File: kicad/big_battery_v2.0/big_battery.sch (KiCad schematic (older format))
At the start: 86 parts, among them J1 CN3, J2 CN2, J3 MCU, J4 P1, J5 P0, J6 PRGM, J7 DI, J8 DO, Q1 AO3400, Q2 AO3400, Q3 AO3400, U1 AP1117-ADJ, U2 LMV324, U3 LMV358, U4 EFM8BB10F2G-A-QFN20, U5 PC817, U6 PC817

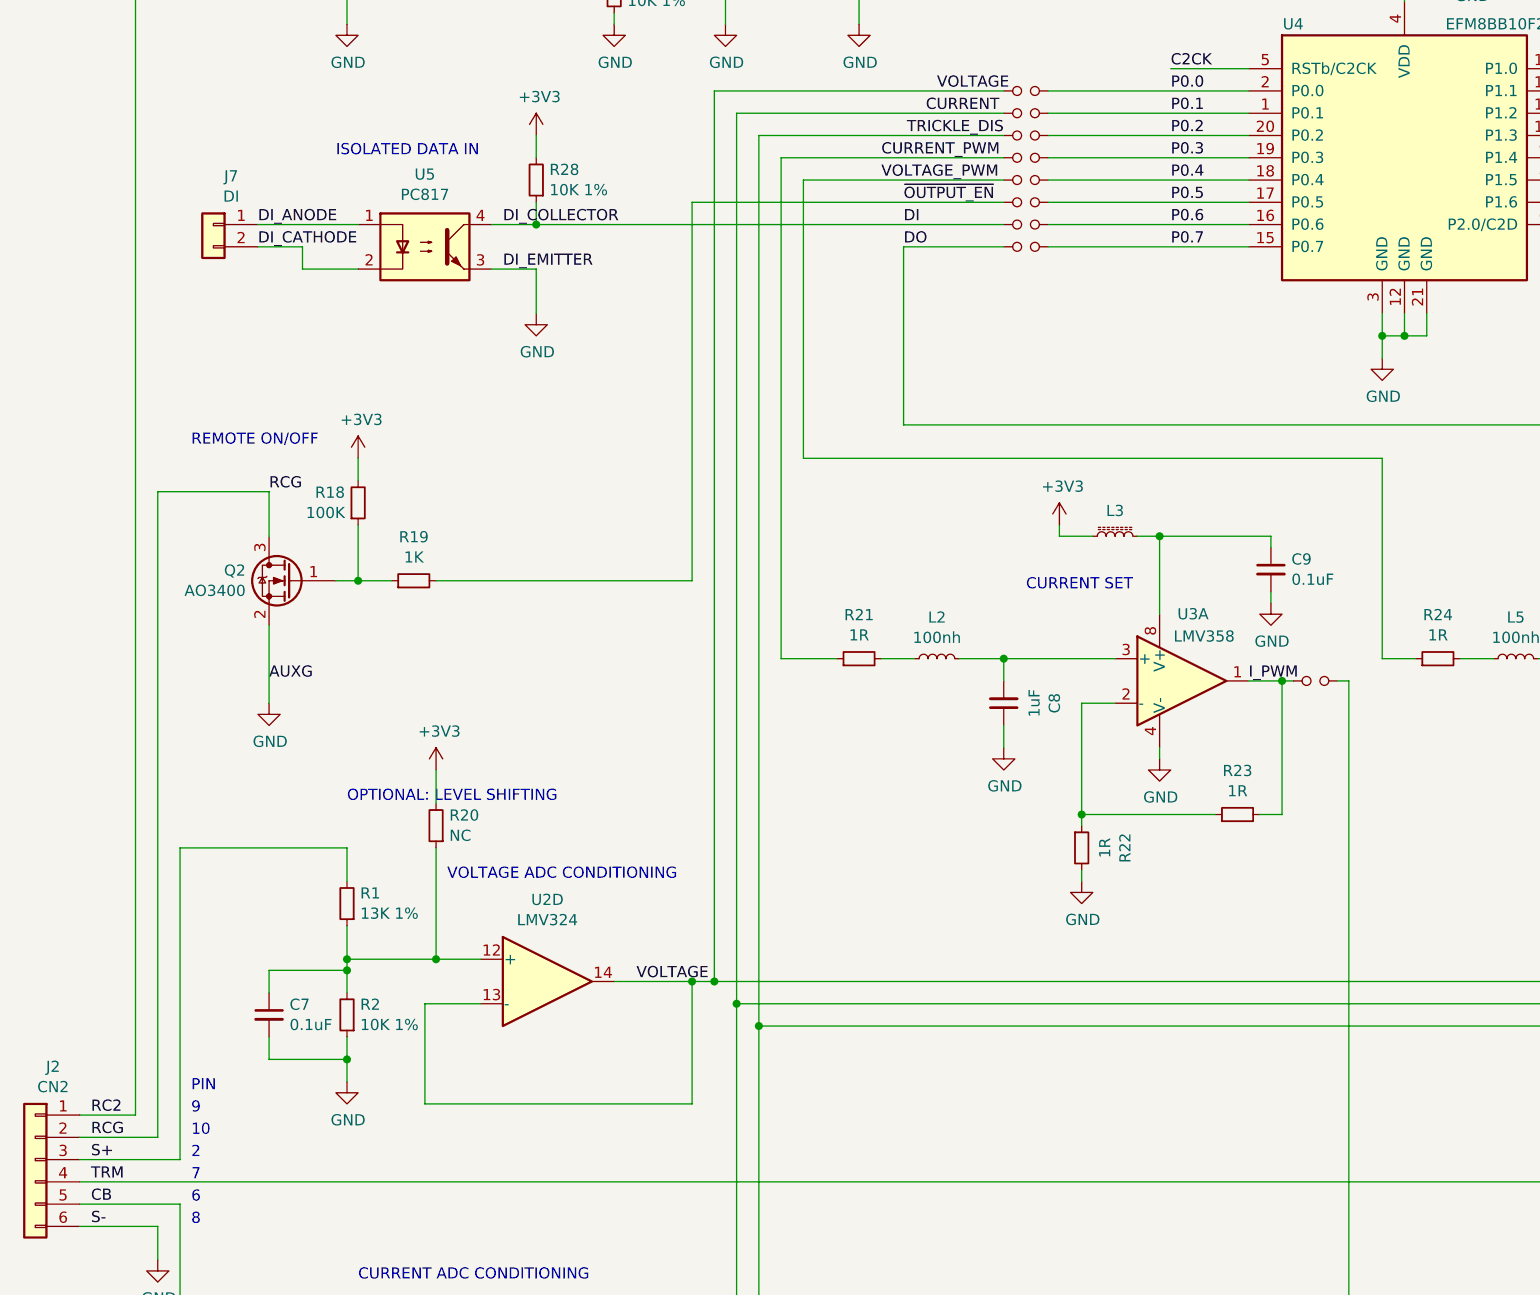
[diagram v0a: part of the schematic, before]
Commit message: final gerbers sent out
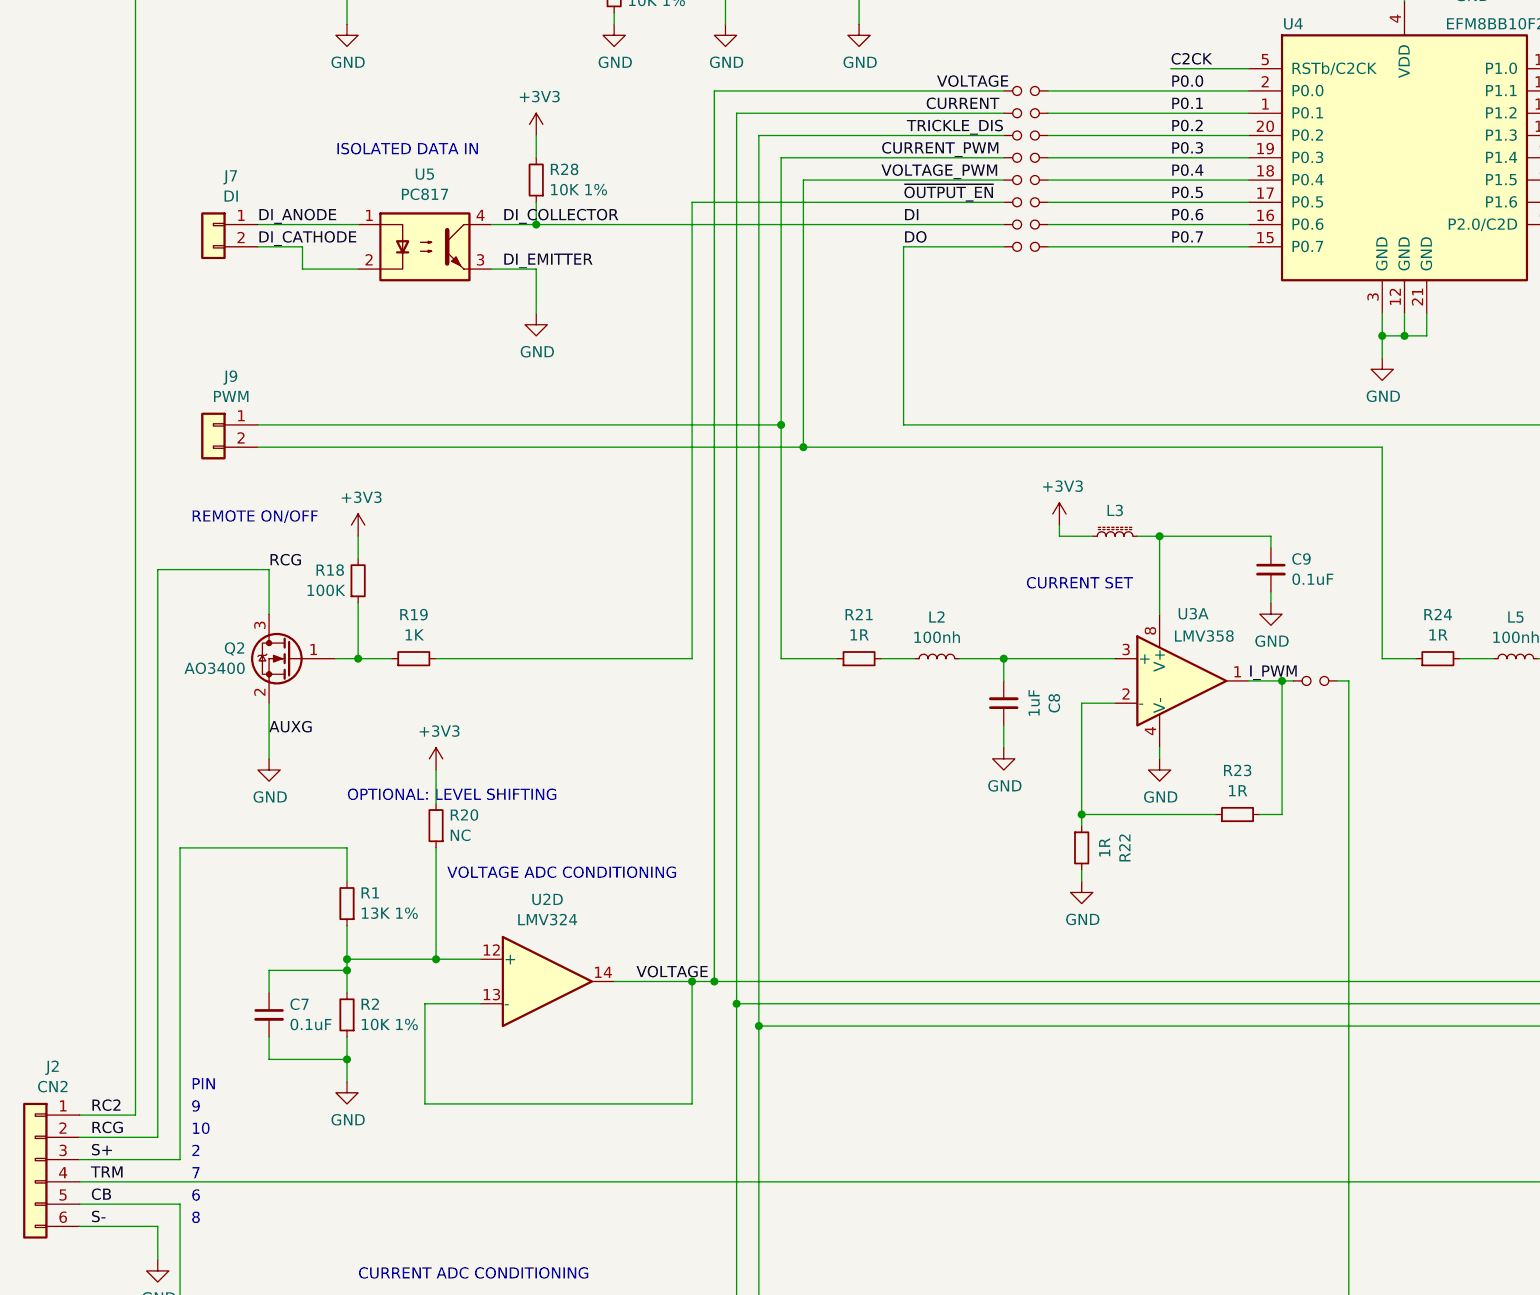
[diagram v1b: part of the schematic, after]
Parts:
- added J9: PWM, Connector_JST:JST_EH_B02B-EH-A_1x02_P2.50mm_Vertical, symbol Connector_Generic:Conn_01x02
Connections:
- net CURRENT_PWM: now also J9.1 (Pin_1)
- net VOLTAGE_PWM: now also J9.2 (Pin_2)
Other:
- moved on the sheet: Q2, R18, R19
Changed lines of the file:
@@
 Connection ~ 4150 6250
 Wire Wire Line
-	4250 2350 4250 4600
+	4250 2350 4250 3550
 Wire Wire Line
 	4250 4600 4500 4600
 Wire Wire Line
-	4350 2450 4350 3700
-Wire Wire Line
-	4350 3700 6950 3700
-Wire Wire Line
-	6950 3700 6950 4600
+	4350 2450 4350 3650
+Wire Wire Line
+	4350 3650 6950 3650
+Wire Wire Line
+	6950 3650 6950 4600
 Wire Wire Line
 	6800 4700 6800 8850
@@
 L big_battery-rescue:Q_NMOS_GSD-Device Q2
 U 1 1 5C8B7C86
-P 2050 4250
-F 0 "Q2" H 2255 4296 50  0000 L CNN
-F 1 "AO3400" H 2255 4205 50  0000 L CNN
-F 2 "Package_TO_SOT_SMD:SOT-23_Handsoldering" H 2250 4350 50  0001 C CNN
-F 3 "~" H 2050 4250 50  0001 C CNN
-	1    2050 4250
+P 2050 4600
+F 0 "Q2" H 2255 4646 50  0000 L CNN
+F 1 "AO3400" H 2255 4555 50  0000 L CNN
+F 2 "Package_TO_SOT_SMD:SOT-23_Handsoldering" H 2250 4700 50  0001 C CNN
+F 3 "~" H 2050 4600 50  0001 C CNN
+	1    2050 4600
 	-1   0    0    -1
 $EndComp
@@
 	1350 1350 1350 6650
 Wire Wire Line
-	1450 3850 1950 3850
-Wire Wire Line
-	1950 3850 1950 4050
-Wire Wire Line
-	1450 3850 1450 6750
+	1450 4200 1950 4200
+Wire Wire Line
+	1950 4200 1950 4400
+Wire Wire Line
+	1450 4200 1450 6750
 $Comp
 L big_battery-rescue:R_Small-Device R19
 U 1 1 5C91C427
-P 2600 4250
-F 0 "R19" V 2796 4250 50  0000 C CNN
-F 1 "1K" V 2705 4250 50  0000 C CNN
-F 2 "Resistor_SMD:R_0603_1608Metric_Pad1.05x0.95mm_HandSolder" H 2600 4250 50  0001 C CNN
-F 3 "~" H 2600 4250 50  0001 C CNN
-	1    2600 4250
+P 2600 4600
+F 0 "R19" V 2796 4600 50  0000 C CNN
+F 1 "1K" V 2705 4600 50  0000 C CNN
+F 2 "Resistor_SMD:R_0603_1608Metric_Pad1.05x0.95mm_HandSolder" H 2600 4600 50  0001 C CNN
+F 3 "~" H 2600 4600 50  0001 C CNN
+	1    2600 4600
 	0    -1   -1   0
 $EndComp
@@
 L big_battery-rescue:R_Small-Device R18
 U 1 1 5C91C717
-P 2350 3900
-F 0 "R18" H 2291 3854 50  0000 R CNN
-F 1 "100K" H 2291 3945 50  0000 R CNN
-F 2 "Resistor_SMD:R_0603_1608Metric_Pad1.05x0.95mm_HandSolder" H 2350 3900 50  0001 C CNN
-F 3 "~" H 2350 3900 50  0001 C CNN
-	1    2350 3900
+P 2350 4250
+F 0 "R18" H 2291 4204 50  0000 R CNN
+F 1 "100K" H 2291 4295 50  0000 R CNN
+F 2 "Resistor_SMD:R_0603_1608Metric_Pad1.05x0.95mm_HandSolder" H 2350 4250 50  0001 C CNN
+F 3 "~" H 2350 4250 50  0001 C CNN
+	1    2350 4250
 	1    0    0    1
 $EndComp
@@
 L big_battery-rescue:GND-power #PWR0120
 U 1 1 5C9461A6
-P 1950 4800
-F 0 "#PWR0120" H 1950 4550 50  0001 C CNN
-F 1 "GND" H 1955 4627 50  0000 C CNN
-F 2 "" H 1950 4800 50  0001 C CNN
-F 3 "" H 1950 4800 50  0001 C CNN
-	1    1950 4800
-	1    0    0    -1
-$EndComp
-Wire Wire Line
-	2250 4250 2350 4250
-Wire Wire Line
-	1950 4450 1950 4800
+P 1950 5050
+F 0 "#PWR0120" H 1950 4800 50  0001 C CNN
+F 1 "GND" H 1955 4877 50  0000 C CNN
+F 2 "" H 1950 5050 50  0001 C CNN
+F 3 "" H 1950 5050 50  0001 C CNN
+	1    1950 5050
+	1    0    0    -1
+$EndComp
+Wire Wire Line
+	2250 4600 2350 4600
+Wire Wire Line
+	1950 4800 1950 5050
 $Comp
 L big_battery-rescue:+3V3-power #PWR0121
 U 1 1 5C971343
-P 2350 3700
-F 0 "#PWR0121" H 2350 3550 50  0001 C CNN
-F 1 "+3V3" H 2365 3873 50  0000 C CNN
-F 2 "" H 2350 3700 50  0001 C CNN
-F 3 "" H 2350 3700 50  0001 C CNN
-	1    2350 3700
-	1    0    0    -1
-$EndComp
-Wire Wire Line
-	2350 3700 2350 3800
-Wire Wire Line
-	2350 4000 2350 4250
-Connection ~ 2350 4250
-Wire Wire Line
-	2350 4250 2500 4250
+P 2350 4050
+F 0 "#PWR0121" H 2350 3900 50  0001 C CNN
+F 1 "+3V3" H 2365 4223 50  0000 C CNN
+F 2 "" H 2350 4050 50  0001 C CNN
+F 3 "" H 2350 4050 50  0001 C CNN
+	1    2350 4050
+	1    0    0    -1
+$EndComp
+Wire Wire Line
+	2350 4050 2350 4150
+Wire Wire Line
+	2350 4350 2350 4600
+Connection ~ 2350 4600
+Wire Wire Line
+	2350 4600 2500 4600
 $Comp
 L Device:Jumper_NO_Small JP7
@@
 	5450 2550 6350 2550
 Wire Wire Line
-	3850 4250 3850 2550
-Wire Wire Line
-	2700 4250 3850 4250
+	3850 4600 3850 2550
+Wire Wire Line
+	2700 4600 3850 4600
 Wire Wire Line
 	3850 2550 5250 2550
@@
 	1    0    0    -1
 $EndComp
-Text Label 1950 4700 0    50   ~ 0
+Text Label 1950 4950 0    50   ~ 0
 AUXG
-Text Label 1950 3850 0    50   ~ 0
+Text Label 1950 4200 0    50   ~ 0
 RCG
 $Comp
@@
 Text Notes 2250 2350 0    50   ~ 0
 ISOLATED DATA IN
-Text Notes 1600 3650 0    50   ~ 0
+Text Notes 1600 4000 0    50   ~ 0
 REMOTE ON/OFF
 Text Notes 1600 6550 0    50   ~ 0
@@
 Text Label 7850 8400 0    50   ~ 0
 I_LIMIT
+$Comp
+L Connector_Generic:Conn_01x02 J9
+U 1 1 5C4891A7
+P 1700 3550
+F 0 "J9" H 1620 3767 50  0000 C CNN
+F 1 "PWM" H 1620 3676 50  0000 C CNN
+F 2 "Connector_JST:JST_EH_B02B-EH-A_1x02_P2.50mm_Vertical" H 1700 3550 50  0001 C CNN
+F 3 "~" H 1700 3550 50  0001 C CNN
+	1    1700 3550
+	-1   0    0    -1
+$EndComp
+Wire Wire Line
+	4350 3650 1900 3650
+Connection ~ 4350 3650
+Wire Wire Line
+	4250 3550 1900 3550
+Connection ~ 4250 3550
+Wire Wire Line
+	4250 3550 4250 4600
 $EndSCHEMATC
